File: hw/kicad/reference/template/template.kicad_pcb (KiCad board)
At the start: 2 copper layers, 40 x 40 mm, 2 parts, among them J1 TOP, J2 BUTTOM

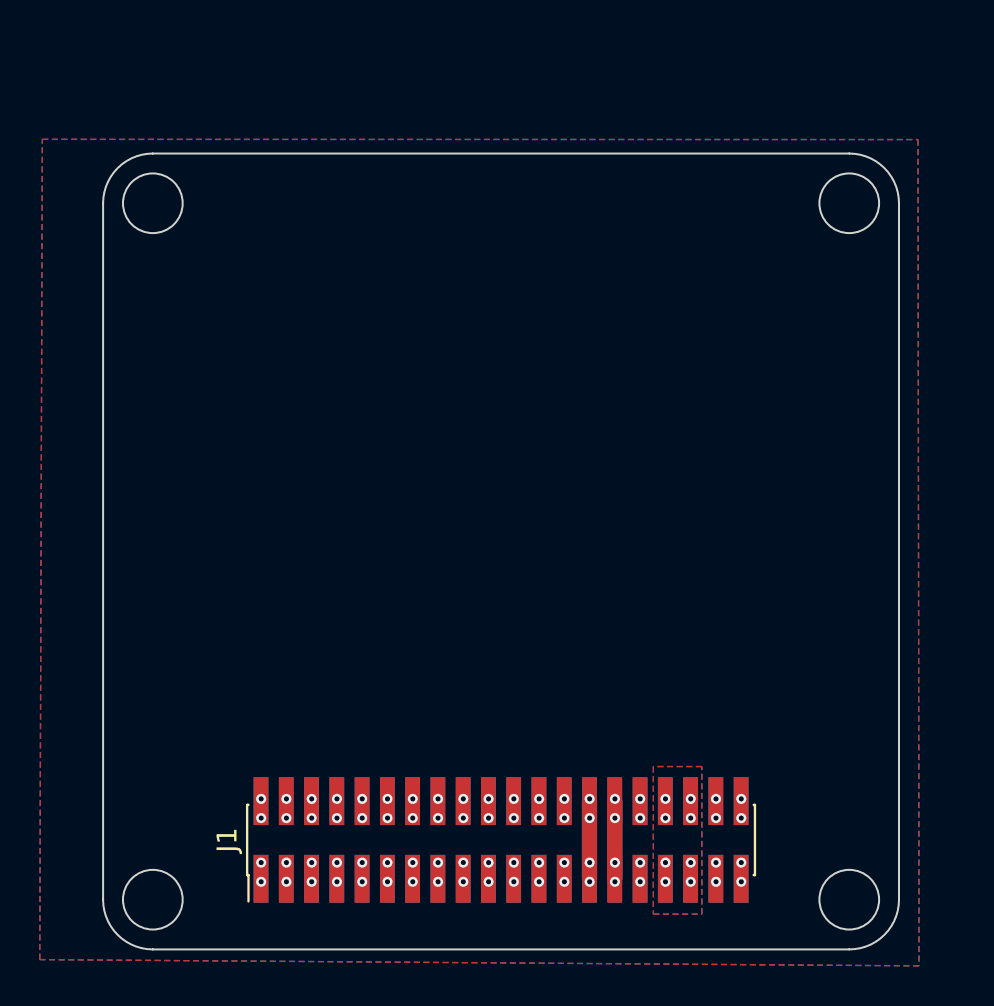
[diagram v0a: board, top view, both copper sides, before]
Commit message: Merge from normal
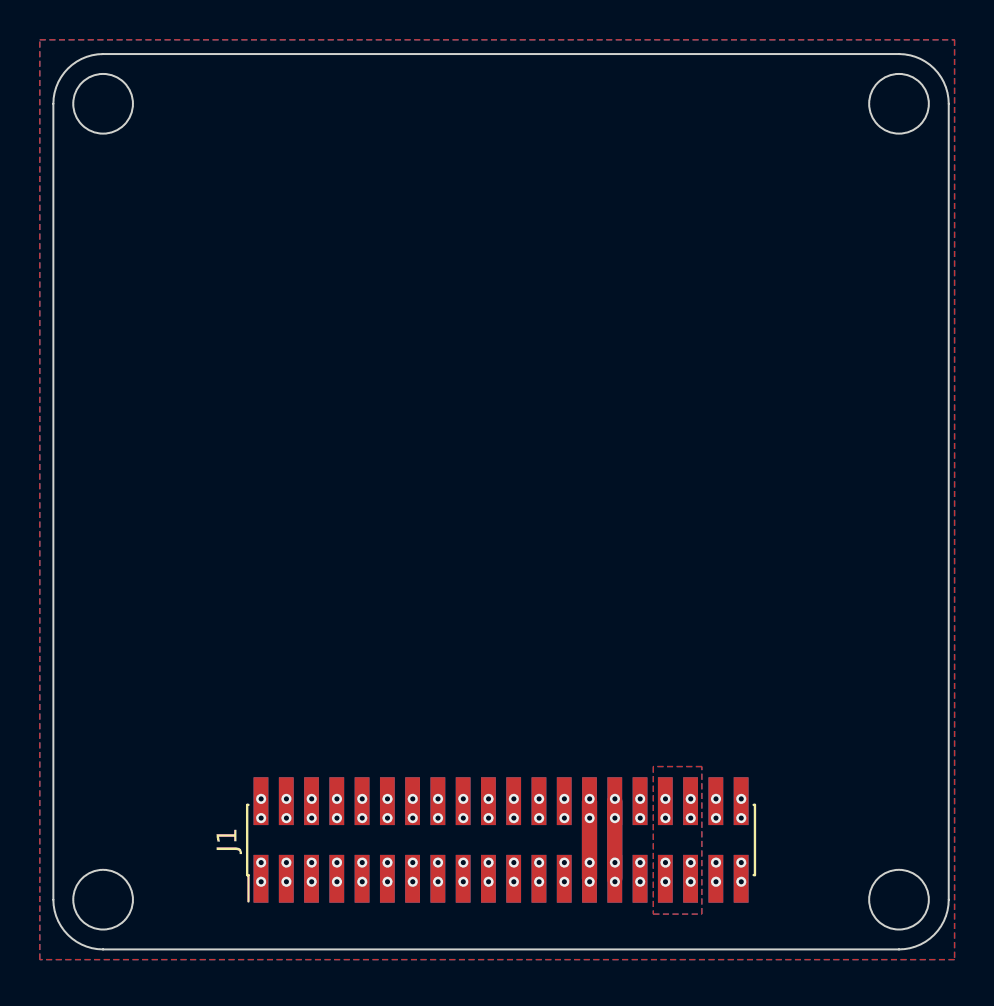
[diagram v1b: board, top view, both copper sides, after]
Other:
- board size 40 x 40 mm -> 45 x 45 mm
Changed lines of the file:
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@@
     )
     (pad_to_mask_clearance 0)
-    (grid_origin 55.72 75.22)
+    (grid_origin 53.22 75.22)
     (pcbplotparams
       (layerselection 0x00010fc_ffffffff)
@@
     )
   )
-  (gr_line locked (start 93.22 75.22) (end 93.22 40.22)
+  (gr_line locked (start 95.72 75.22) (end 95.72 35.22)
     (stroke (width 0.1) (type default)) (layer "Edge.Cuts"))
-  (gr_arc locked (start 53.22 40.22) (mid 53.952233 38.452233) (end 55.72 37.72)
+  (gr_arc locked (start 50.72 35.22) (mid 51.452233 33.452233) (end 53.22 32.72)
     (stroke (width 0.1) (type default)) (layer "Edge.Cuts"))
-  (gr_circle locked (center 90.72 75.22) (end 89.22 75.22)
+  (gr_circle locked (center 93.22 75.22) (end 91.72 75.22)
     (stroke (width 0.1) (type default)) (fill none) (layer "Edge.Cuts"))
-  (gr_circle locked (center 55.72 40.22) (end 57.22 40.22)
+  (gr_circle locked (center 53.22 35.22) (end 54.72 35.22)
     (stroke (width 0.1) (type default)) (fill none) (layer "Edge.Cuts"))
-  (gr_line locked (start 90.72 37.72) (end 55.72 37.72)
+  (gr_line locked (start 93.22 32.72) (end 53.22 32.72)
     (stroke (width 0.1) (type default)) (layer "Edge.Cuts"))
-  (gr_arc locked (start 90.72 37.72) (mid 92.487767 38.452233) (end 93.22 40.22)
+  (gr_arc locked (start 93.22 32.72) (mid 94.987767 33.452233) (end 95.72 35.22)
     (stroke (width 0.1) (type default)) (layer "Edge.Cuts"))
-  (gr_arc locked (start 93.22 75.22) (mid 92.487767 76.987767) (end 90.72 77.72)
+  (gr_arc locked (start 95.72 75.22) (mid 94.987767 76.987767) (end 93.22 77.72)
     (stroke (width 0.1) (type default)) (layer "Edge.Cuts"))
-  (gr_circle locked (center 90.72 40.22) (end 90.72 41.72)
+  (gr_circle locked (center 93.22 35.22) (end 93.22 36.72)
     (stroke (width 0.1) (type default)) (fill none) (layer "Edge.Cuts"))
-  (gr_line locked (start 55.72 77.72) (end 90.72 77.72)
+  (gr_line locked (start 53.22 77.72) (end 93.22 77.72)
     (stroke (width 0.1) (type default)) (layer "Edge.Cuts"))
-  (gr_arc locked (start 55.72 77.72) (mid 53.952233 76.987767) (end 53.22 75.22)
+  (gr_arc locked (start 53.22 77.72) (mid 51.452233 76.987767) (end 50.72 75.22)
     (stroke (width 0.1) (type default)) (layer "Edge.Cuts"))
-  (gr_circle locked (center 55.72 75.22) (end 55.72 73.72)
+  (gr_circle locked (center 53.22 75.22) (end 53.22 73.72)
     (stroke (width 0.1) (type default)) (fill none) (layer "Edge.Cuts"))
-  (gr_line locked (start 53.22 40.22) (end 53.22 75.22)
+  (gr_line locked (start 50.72 35.22) (end 50.72 75.22)
     (stroke (width 0.1) (type default)) (layer "Edge.Cuts"))
   (segment (start 77.665 70.27) (end 77.665 74.17) (width 0.762) (layer "F.Cu") (net 1))
@@
     (connect_pads yes (clearance 0.1524))
     (min_thickness 0.1524) (filled_areas_thickness no)
-    (fill (thermal_gap 0.1524) (thermal_bridge_width 0.1524) (smoothing fillet) (radius 0.1524))
+    (fill yes (thermal_gap 0.1524) (thermal_bridge_width 0.1524) (smoothing fillet) (radius 0.1524))
     (polygon
       (pts
-        (xy 50.165 37.0078)
-        (xy 94.1756 37.0184)
-        (xy 94.2264 78.5474)
+        (xy 50.038 32.004)
+        (xy 96.012 32.004)
+        (xy 96.012 78.232)
         (xy 50.038 78.232)
       )
